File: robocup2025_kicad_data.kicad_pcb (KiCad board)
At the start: 4 copper layers, 15 parts, among them M7 Motor_Servo, U2 ESP32-DEVKITC-32E

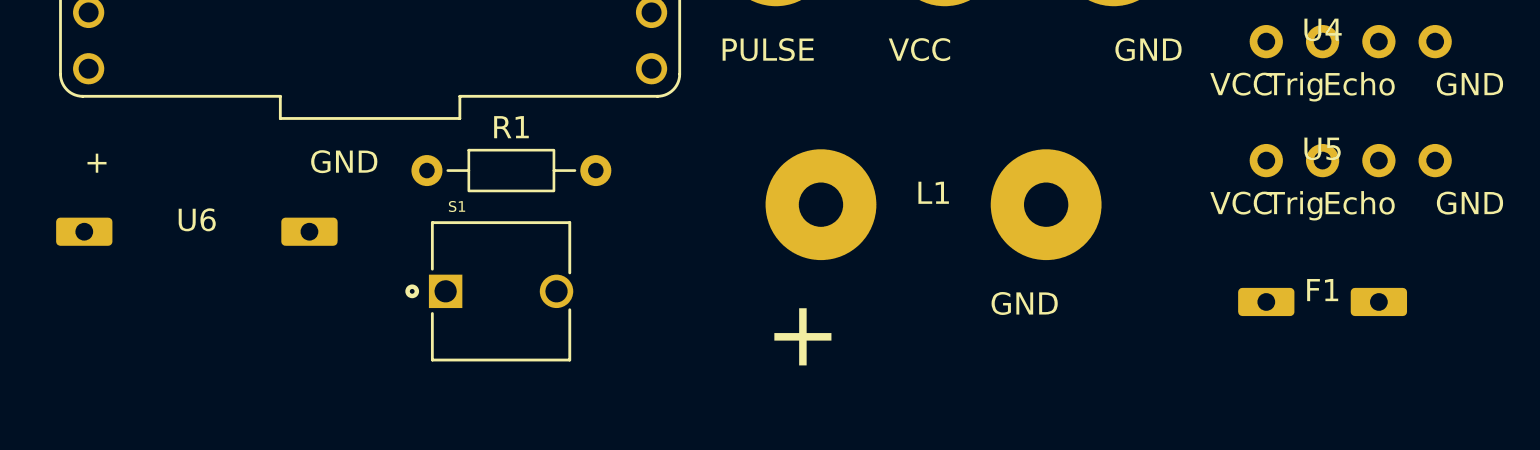
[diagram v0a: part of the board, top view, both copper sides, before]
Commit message: changed place
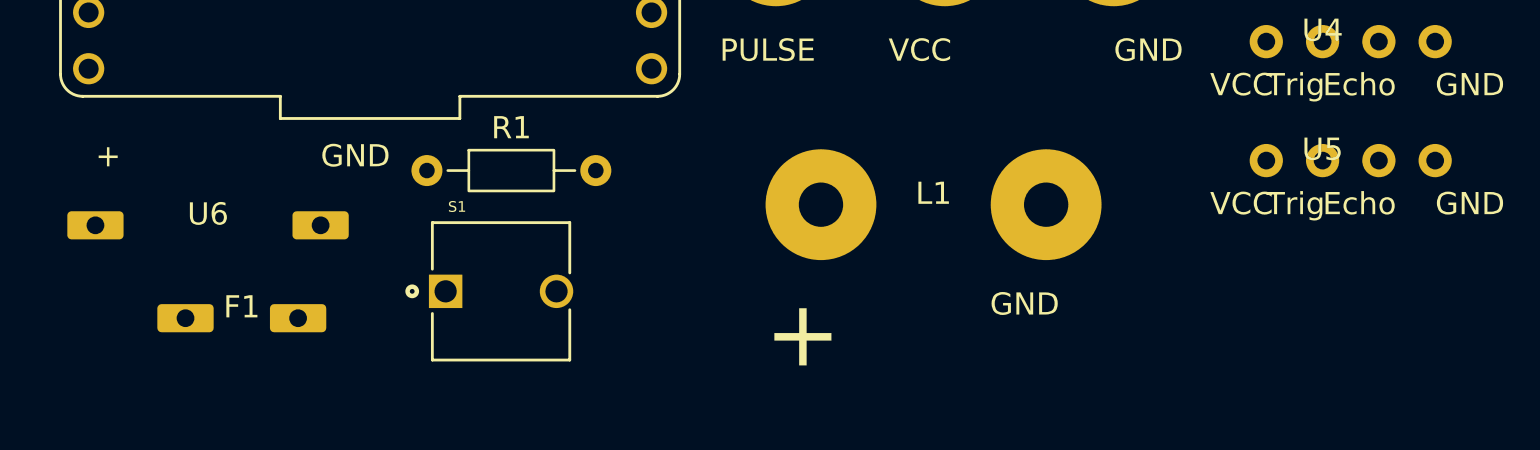
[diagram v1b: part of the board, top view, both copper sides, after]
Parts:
- moved F1 48.8 mm to (142.0, 117.6)
- moved U6 0.58 mm to (140.5, 113.4)
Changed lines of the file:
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@@
 	(footprint "robo:voltmeter"
 		(layer "F.Cu")
-		(at 139.958 113.7)
+		(at 140.462 113.411)
 		(property "Reference" "U6"
 			(at 0 -0.5 0)
@@
 	(footprint "robo:fuse_holder"
 		(layer "F.Cu")
-		(at 190.754 116.87)
+		(at 141.986 117.602)
 		(property "Reference" "F1"
 			(at 0 -0.5 0)
